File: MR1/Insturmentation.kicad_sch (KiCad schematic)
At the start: 45 parts, among them J1 Conn_01x01_Pin, J10 Conn_01x01_Pin, J11 Conn_01x01_Pin, J12 Conn_01x10, J13 Conn_01x10, J14 Conn_01x10, J2 Conn_01x01_Pin, J9 Conn_01x10, U10 AD40xxBRMZ, U11 LP5907MFX-1.8, U16 LTC6268xS8, U2 LMP7721, U6 ADA4940-1xCP

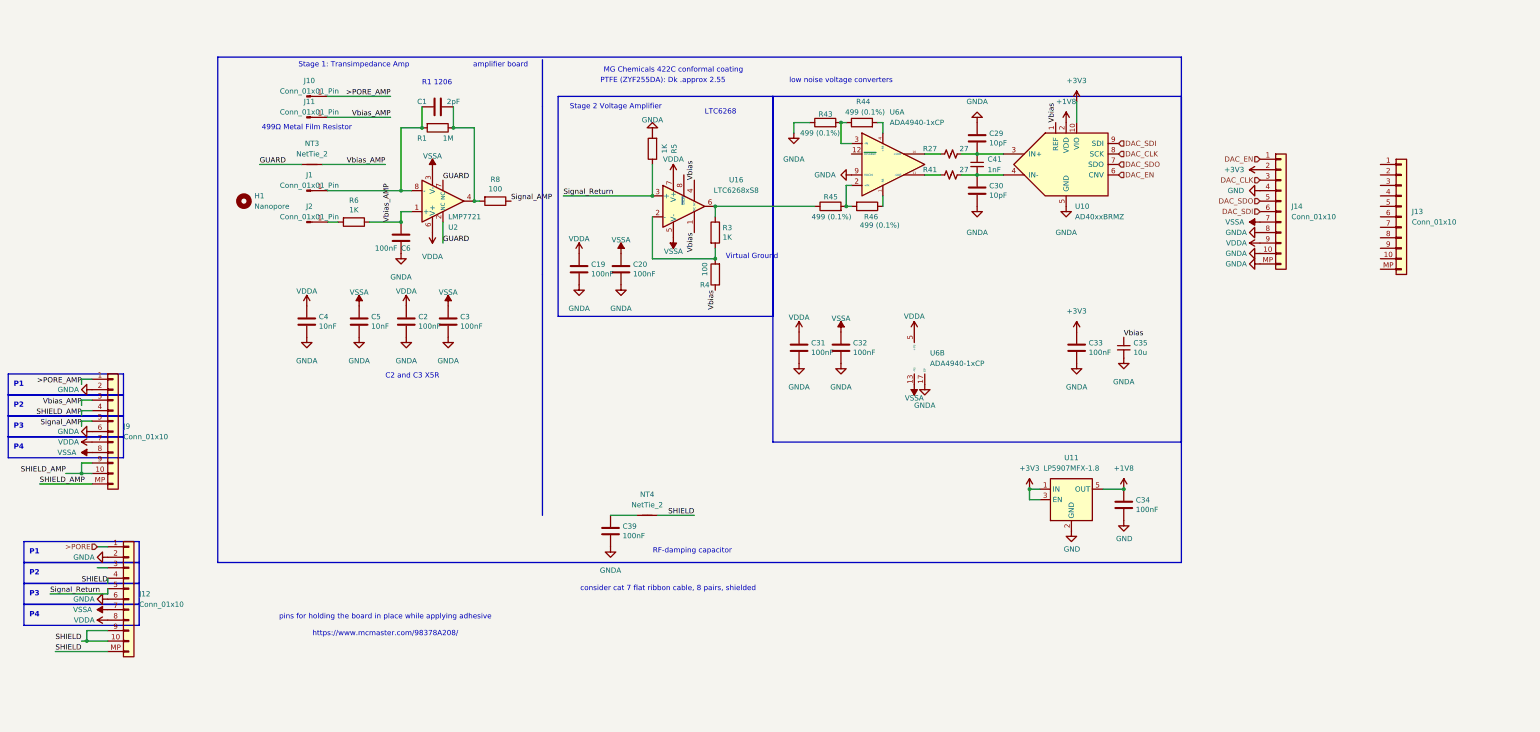
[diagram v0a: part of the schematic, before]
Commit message: commiting pcb changes
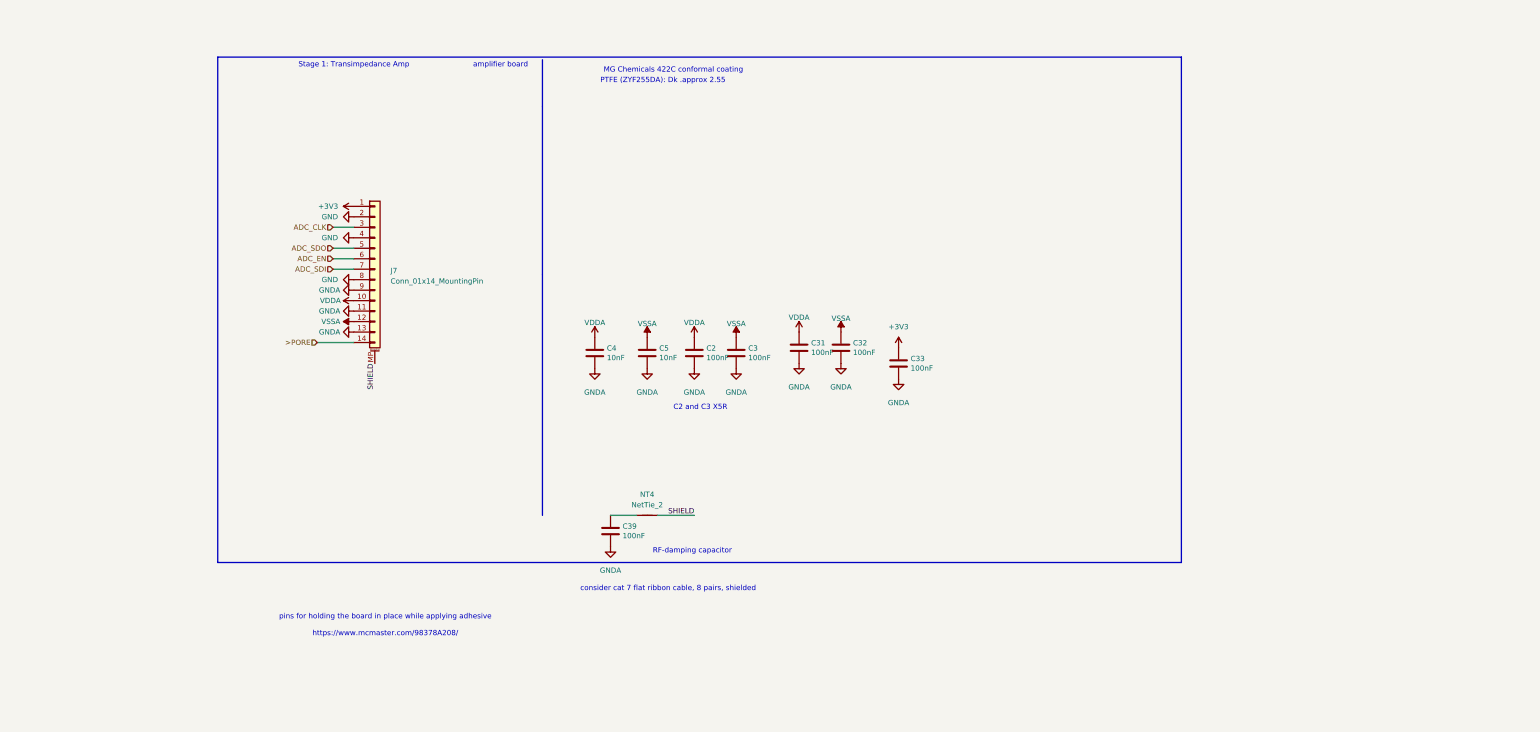
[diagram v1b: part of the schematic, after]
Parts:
- removed C1: 2pF, Capacitor_SMD:C_0402_1005Metric, symbol Device:C
- removed C19, C20, C34, C6: 100nF, Capacitor_SMD:C_0402_1005Metric, symbol Device:C
- removed C29, C30: 10pF, Capacitor_SMD:C_0402_1005Metric, symbol Device:C
- removed C35: 10u, Capacitor_SMD:C_0402_1005Metric, symbol Device:C_Small
- removed C41: 1nF, Capacitor_SMD:C_0402_1005Metric, symbol Device:C_Small
- removed H1: Nanopore, footprints:Nanopore holder_recessed, symbol Mechanical:MountingHole
- removed J1, J10, J11, J2: Conn_01x01_Pin, footprints:Electrode, symbol Connector:Conn_01x01_Pin
- removed J12, J13, J14, J9: Conn_01x10, Connector_JST:JST_SH_SM10B-SRSS-TB_1x10-1MP_P1.00mm_Horizontal, symbol MR1:Conn_01x11_MP
- removed NT3: NetTie_2, NetTie:NetTie-2_SMD_Pad0.5mm, symbol Device:NetTie_2
- removed R1: 1M, Resistor_SMD:R_0402_1005Metric, symbol Device:R
- removed R27, R41: 27, Resistor_SMD:R_0402_1005Metric, symbol Device:R_Small_US
- removed R3, R5, R6: 1K, Resistor_SMD:R_0402_1005Metric, symbol Device:R
- removed R4, R8: 100, Resistor_SMD:R_0402_1005Metric, symbol Device:R
- removed R43, R44, R45, R46: 499 (0.1%), Resistor_SMD:R_0402_1005Metric, symbol Device:R
- removed U10: AD40xxBRMZ, Package_SO:MSOP-10_3x3mm_P0.5mm, symbol Analog_ADC:AD40xxBRMZ
- removed U11: LP5907MFX-1.8, Package_TO_SOT_SMD:SOT-23-5, symbol Regulator_Linear:LP5907MFX-1.8
- removed U16: LTC6268xS8, Package_SO:SO-8_3.9x4.9mm_P1.27mm, symbol MR1:LTC6268xS8-10_SHIELD
- removed U2: LMP7721, Package_SO:SOIC-8_3.9x4.9mm_P1.27mm, symbol LMP7721:LMP7721
- removed U6: ADA4940-1xCP, Package_CSP:LFCSP-16-1EP_3x3mm_P0.5mm_EP1.3x1.3mm_ThermalVias, symbol Amplifier_Difference:ADA4940-1xCP
- added J7: Conn_01x14_MountingPin, Connector_FFC-FPC:Amphenol_F32R-1A7x1-11014_1x14-1MP_P0.5mm_Horizontal, symbol Connector_Generic_MountingPin:Conn_01x14_MountingPin
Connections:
- net +3V3: now also J7.1 (Pin_1)
- net >PORE: now also J7.14 (Pin_14)
- net GND: now also J7.2 (Pin_2), J7.4 (Pin_4), J7.8 (Pin_8)
- net GNDA: now also J7.11 (Pin_11), J7.13 (Pin_13), J7.9 (Pin_9)
- net SHIELD: now also J7.MP (MountPin)
- net VDDA: now also J7.10 (Pin_10)
- net VSSA: now also J7.12 (Pin_12)
- new net ADC_CLK: J7.3 (Pin_3)
- new net ADC_EN: J7.6 (Pin_6)
- new net ADC_SDI: J7.7 (Pin_7)
- new net ADC_SDO: J7.5 (Pin_5)
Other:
- note removed: "499Ω Metal Film Resistor"
- note removed: "LTC6268"
- note removed: "P1"
- note removed: "P2"
- note removed: "P3"
- note removed: "P4"
- note removed: "R1 1206"
- note removed: "Stage 2 Voltage Amplifier"
- note removed: "Virtual Ground"
- note removed: "low noise voltage converters"
- moved on the sheet: C2, C3, C33, C4, C5
